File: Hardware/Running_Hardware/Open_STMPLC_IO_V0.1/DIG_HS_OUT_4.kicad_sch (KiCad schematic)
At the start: 24 parts, among them J15 Screw_Terminal_01x02, Q4 2N7002K, U18 TPS26600PWP, U19 NVTFS5124PLTAG

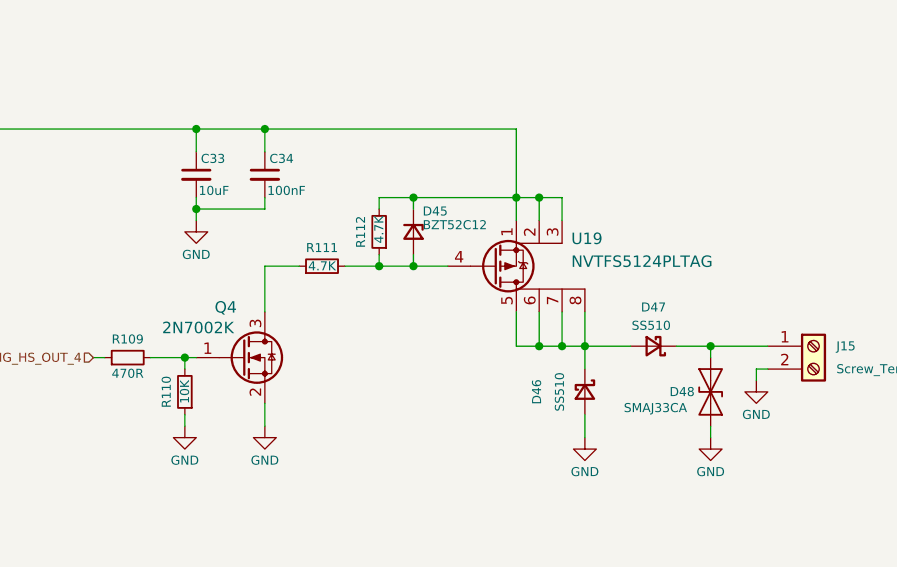
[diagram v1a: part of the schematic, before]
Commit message: Analog input section
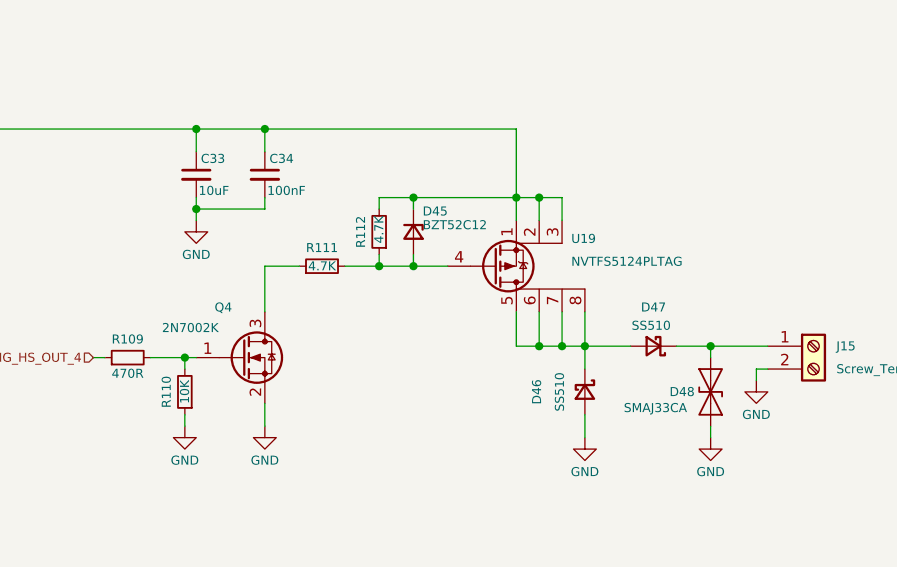
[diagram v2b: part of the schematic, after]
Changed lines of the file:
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@@
 			(effects
 				(font
-					(size 1.27 1.27)
+					(size 1 1)
 				)
 				(justify left)
@@
 			(effects
 				(font
-					(size 1.27 1.27)
+					(size 1 1)
 				)
 				(justify left)
@@
 			(effects
 				(font
-					(size 1.27 1.27)
+					(size 1 1)
 				)
 				(justify left)
@@
 			(effects
 				(font
-					(size 1.27 1.27)
+					(size 1 1)
 				)
 				(justify left)
